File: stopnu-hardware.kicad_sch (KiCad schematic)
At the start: 10 parts, among them CN1 SM04B-SRSS-TB (LF)(SN), CN2 OQ0232510000G, CN3 OQ0232510000G, CN4 OQ0232510000G, CN5 OQ0232510000G, CN6 OQ0432510000G

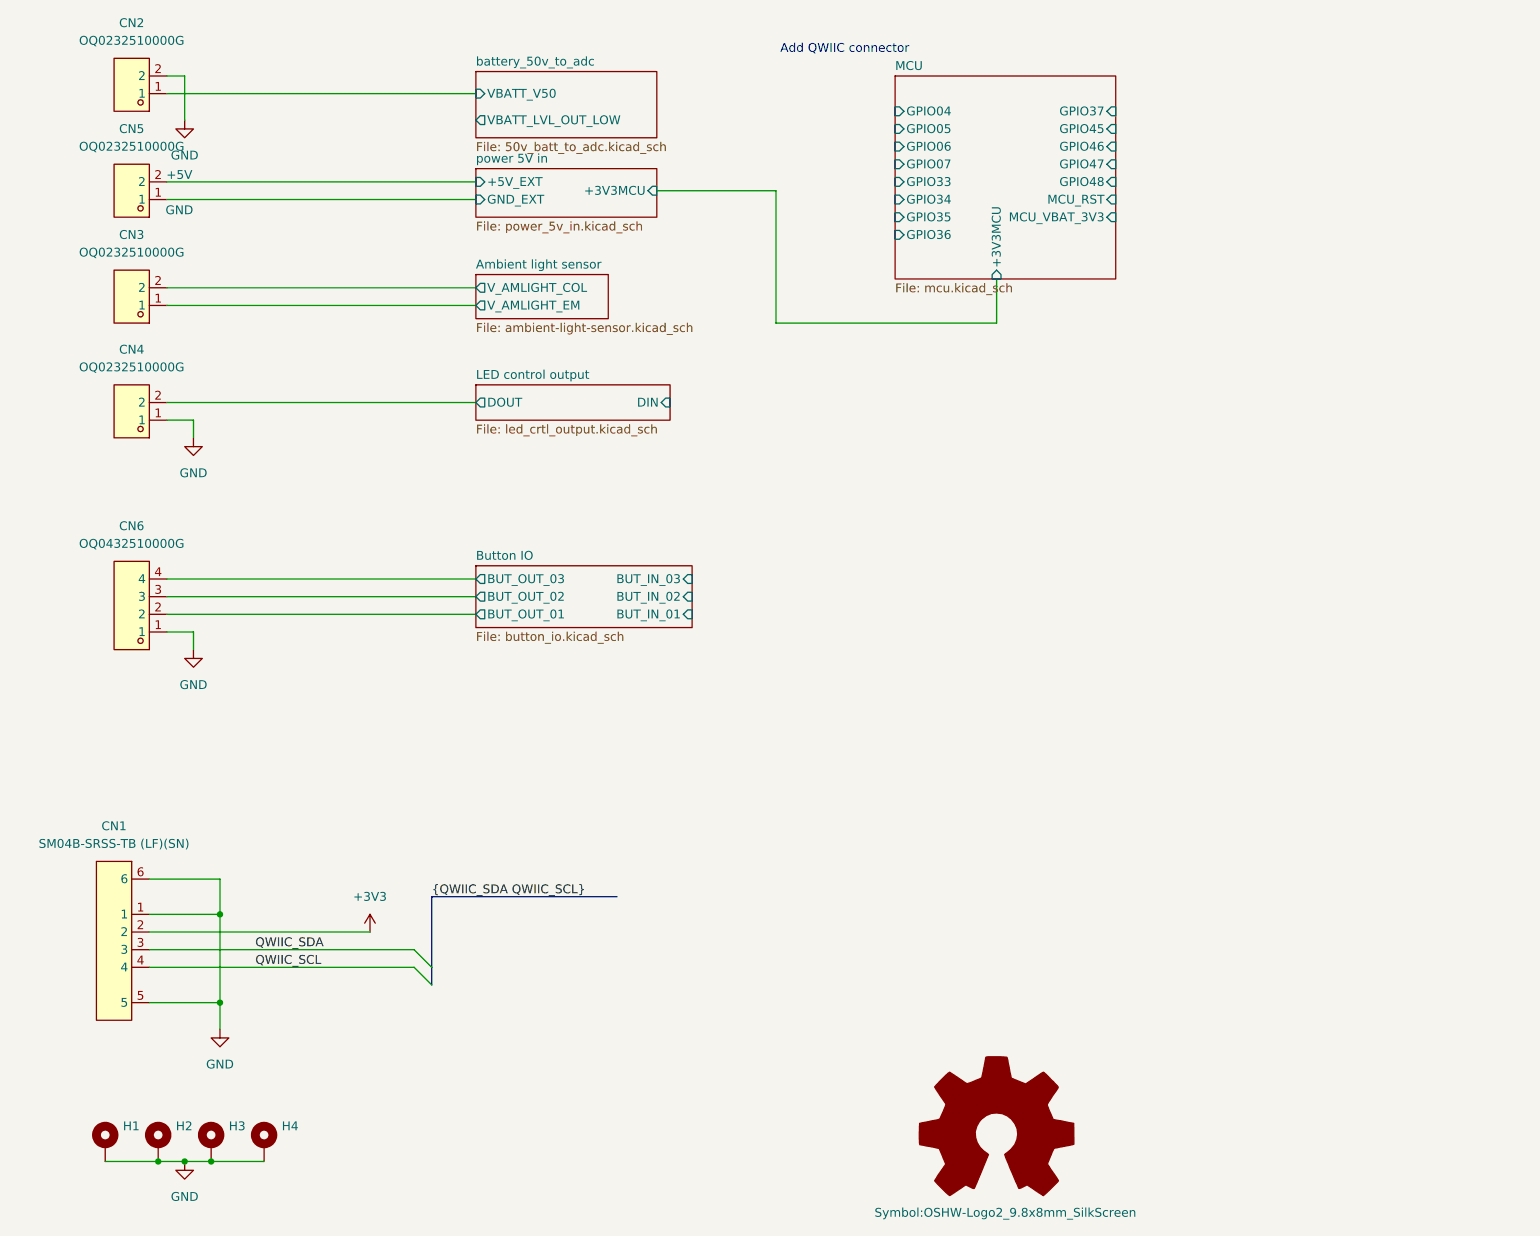
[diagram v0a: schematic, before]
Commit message: Some extra work for building the rats nest.
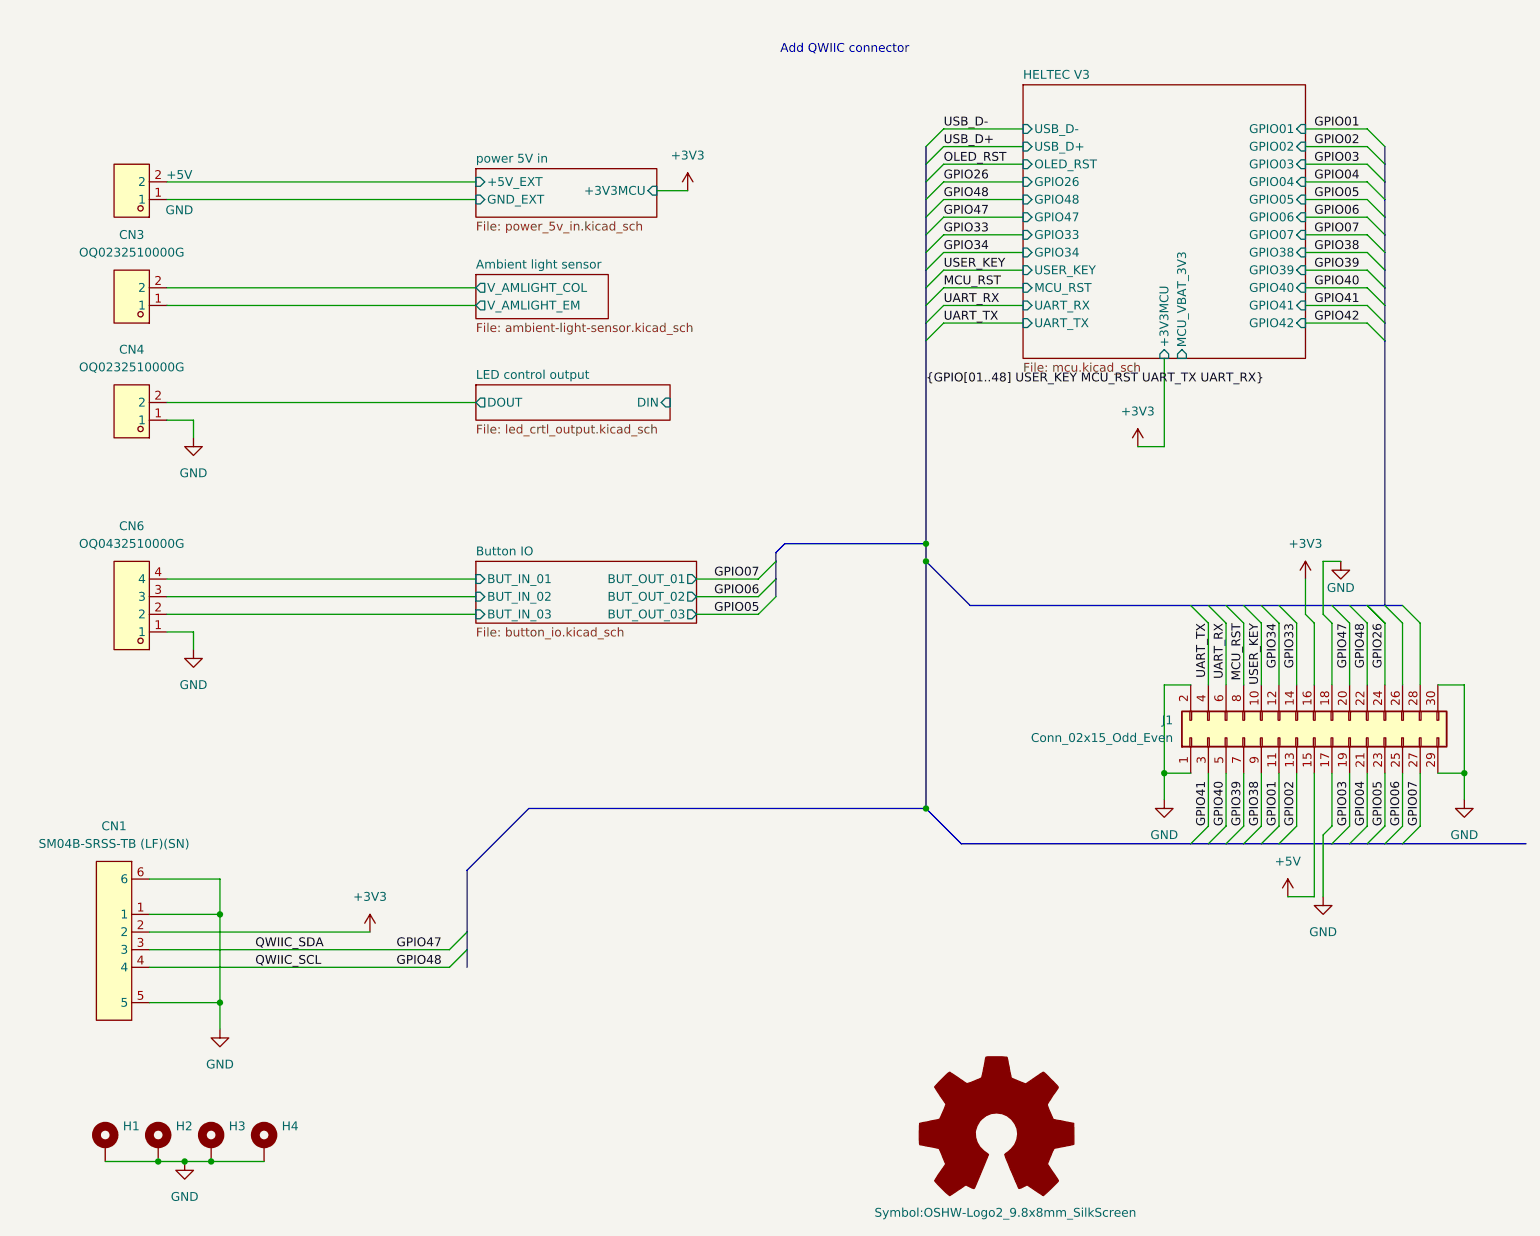
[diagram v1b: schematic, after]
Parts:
- removed CN2: OQ0232510000G, lcsc:CONN-TH_OQ0232510000G, symbol lcsc:OQ0232510000G
- added J1: Conn_02x15_Odd_Even, Connector_PinHeader_2.54mm:PinHeader_2x15_P2.54mm_Horizontal, symbol Connector_Generic:Conn_02x15_Odd_Even
- H1, H2, H3, H4: footprint MountingHole:MountingHole_6mm_Pad -> MountingHole:MountingHole_6.4mm_M6_DIN965_Pad
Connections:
- net Button IO/BUT_OUT_01 is gone; now on net Button IO/BUT_IN_03: CN6.2
- net Button IO/BUT_OUT_02 is gone; now on net Button IO/BUT_IN_02: CN6.3
- net Button IO/BUT_OUT_03 is gone; now on net Button IO/BUT_IN_01: CN6.4
- net +3V3: now also J1.16 (Pin_16)
- net GND: now also J1.1 (Pin_1), J1.17 (Pin_17), J1.18 (Pin_18), J1.2 (Pin_2), J1.29 (Pin_29), J1.30 (Pin_30)
- net QWIIC_SCL renamed GPIO48
- net GPIO48: now also J1.22 (Pin_22)
- net QWIIC_SDA renamed GPIO47
- net GPIO47: now also J1.20 (Pin_20)
- new net +5V: J1.15 (Pin_15)
- new net GPIO01: J1.11 (Pin_11)
- new net GPIO02: J1.13 (Pin_13)
- new net GPIO03: J1.19 (Pin_19)
- new net GPIO04: J1.21 (Pin_21)
- new net GPIO05: J1.23 (Pin_23)
- new net GPIO06: J1.25 (Pin_25)
- new net GPIO07: J1.27 (Pin_27)
- new net GPIO26: J1.24 (Pin_24)
- new net GPIO33: J1.14 (Pin_14)
- new net GPIO34: J1.12 (Pin_12)
- new net GPIO38: J1.9 (Pin_9)
- new net GPIO39: J1.7 (Pin_7)
- new net GPIO40: J1.5 (Pin_5)
- new net GPIO41: J1.3 (Pin_3)
- new net MCU_RST: J1.8 (Pin_8)
- new net UART_RX: J1.6 (Pin_6)
- new net UART_TX: J1.4 (Pin_4)
- new net USER_KEY: J1.10 (Pin_10)
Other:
- sheet MCU renamed HELTEC V3
- removed sheet battery_50v_to_adc
- sheet HELTEC V3 ports: added GPIO01, GPIO02, GPIO03, GPIO26, GPIO38, GPIO39, GPIO40, GPIO41, GPIO42, OLED_RST, UART_RX, UART_TX, USB_D+, USB_D-, USER_KEY; removed GPIO35, GPIO36, GPIO37, GPIO45, GPIO46
